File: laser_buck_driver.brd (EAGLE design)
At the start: 160 x 100 mm, 23 parts, among them IC1 LM358D, IC2 LM2576, SW1 TACT

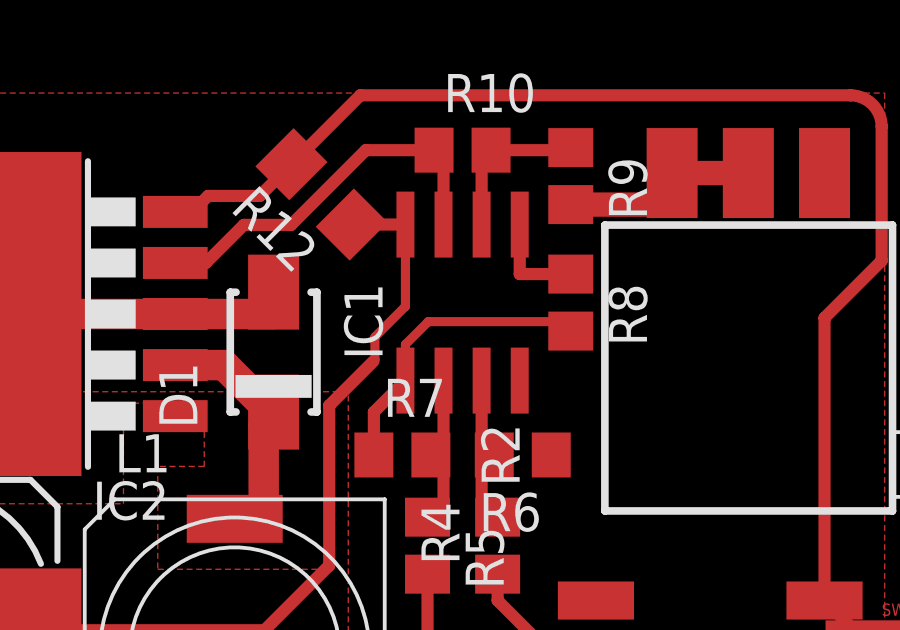
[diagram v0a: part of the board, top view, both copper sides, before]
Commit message: comments
screenshot and minor updates
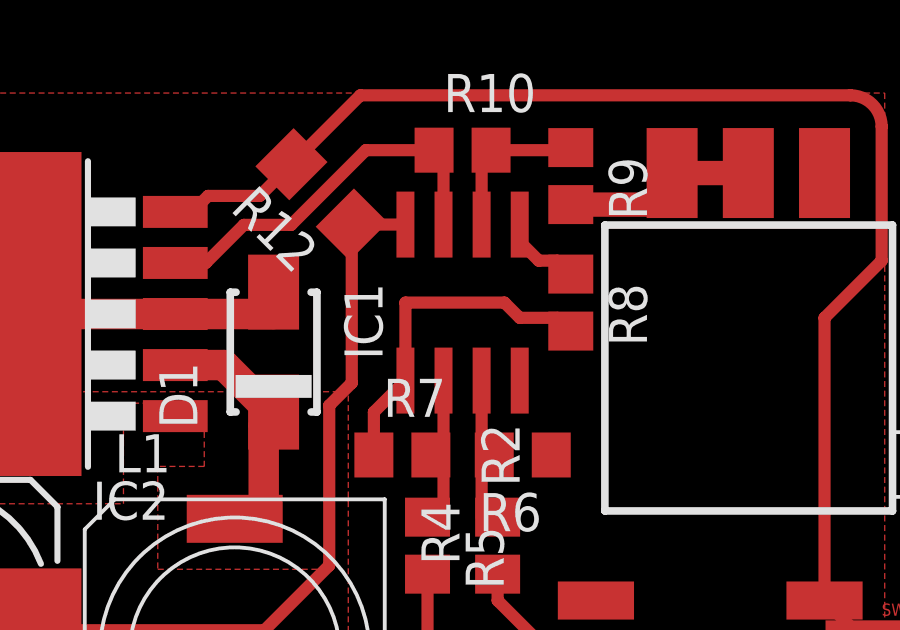
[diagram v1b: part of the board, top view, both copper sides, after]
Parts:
- R10: value 100k -> 470k
- R4, R5: value 22k -> 100k
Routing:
- net N$3: track 10.3 -> 11.7 mm
- net +18V: track 34.5 -> 33.7 mm
- net 22K: track 3.35 -> 2.72 mm
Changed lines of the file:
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@@
 <layer number="23" name="tOrigins" color="15" fill="1" visible="yes" active="yes"/>
 <layer number="24" name="bOrigins" color="15" fill="1" visible="yes" active="yes"/>
-<layer number="25" name="tNames" color="7" fill="1" visible="yes" active="yes"/>
-<layer number="26" name="bNames" color="7" fill="1" visible="yes" active="yes"/>
-<layer number="27" name="tValues" color="7" fill="1" visible="yes" active="yes"/>
-<layer number="28" name="bValues" color="7" fill="1" visible="yes" active="yes"/>
+<layer number="25" name="tNames" color="7" fill="1" visible="no" active="yes"/>
+<layer number="26" name="bNames" color="7" fill="1" visible="no" active="yes"/>
+<layer number="27" name="tValues" color="7" fill="1" visible="no" active="yes"/>
+<layer number="28" name="bValues" color="7" fill="1" visible="no" active="yes"/>
 <layer number="29" name="tStop" color="7" fill="3" visible="no" active="yes"/>
 <layer number="30" name="bStop" color="7" fill="6" visible="no" active="yes"/>
@@
 <rectangle x1="40.259" y1="41.1734" x2="43.6118" y2="44.0436" layer="41"/>
 <rectangle x1="35.179" y1="41.1734" x2="38.5318" y2="44.0436" layer="41"/>
-<dimension x1="71.5264" y1="66.675" x2="71.5264" y2="40.005" x3="78.105" y3="53.34" textsize="1.778" layer="51" dtype="vertical"/>
-<dimension x1="71.5264" y1="40.005" x2="31.6992" y2="40.005" x3="51.6128" y3="33.02" textsize="1.778" layer="51" dtype="vertical"/>
+<dimension x1="71.5264" y1="66.675" x2="71.5264" y2="40.005" x3="74.93" y3="53.34" textsize="1.778" layer="51" dtype="vertical"/>
+<dimension x1="71.5264" y1="40.005" x2="31.6992" y2="40.005" x3="51.6128" y3="36.83" textsize="1.778" layer="51" dtype="vertical"/>
 <wire x1="36.1188" y1="48.7934" x2="38.3286" y2="48.7934" width="0.3048" layer="41"/>
 </plain>
@@
 <element name="C2" library="rcl" package="153CLV-0810" value="100u/25V" x="38.1762" y="49.4538"/>
 <element name="R3" library="rcl" package="R1206" value="0.1R" x="56.8706" y="44.958" rot="R90"/>
-<element name="R4" library="rcl" package="R0805" value="22k" x="57.0484" y="51.4604" rot="R90"/>
-<element name="R5" library="rcl" package="R0805" value="22k" x="54.7116" y="51.4604" rot="R270"/>
+<element name="R4" library="rcl" package="R0805" value="100k" x="57.0484" y="51.4604" rot="R90"/>
+<element name="R5" library="rcl" package="R0805" value="100k" x="54.7116" y="51.4604" rot="R270"/>
 <element name="R6" library="rcl" package="R0805" value="100k" x="57.8866" y="54.483" rot="R180"/>
 <element name="R7" library="rcl" package="R0805" value="100k" x="53.8734" y="54.483"/>
 <element name="R8" library="rcl" package="R0805" value="20k/do_pominiecia" x="59.4868" y="59.563" rot="R270"/>
 <element name="R9" library="rcl" package="R0805" value="1k" x="59.4868" y="63.7794" rot="R270"/>
-<element name="R10" library="rcl" package="R0805" value="100k" x="55.88" y="64.643"/>
+<element name="R10" library="rcl" package="R0805" value="470k" x="55.88" y="64.643"/>
 <element name="SW1" library="miscrel" package="TACT" value="TACT" x="64.135" y="47.0916" rot="R90"/>
 <element name="R12" library="resistor" package="R1206" value="100k" x="51.181" y="63.1698" rot="R135"/>
@@
 <wire x1="52.9234" y1="55.9114" x2="52.9234" y2="54.483" width="0.4064" layer="1"/>
 <wire x1="59.4868" y1="58.928" x2="59.4868" y2="58.613" width="0.3048" layer="1"/>
-<wire x1="54.737" y1="58.928" x2="53.975" y2="58.166" width="0.3048" layer="1"/>
-<wire x1="53.975" y1="58.166" x2="53.975" y2="56.963" width="0.3048" layer="1"/>
-<wire x1="59.4868" y1="58.928" x2="54.737" y2="58.928" width="0.3048" layer="1"/>
+<wire x1="53.975" y1="56.963" x2="53.975" y2="59.563" width="0.4064" layer="1"/>
+<wire x1="53.975" y1="59.563" x2="57.277" y2="59.563" width="0.4064" layer="1"/>
+<wire x1="57.277" y1="59.563" x2="57.785" y2="59.055" width="0.4064" layer="1"/>
+<wire x1="57.785" y1="59.055" x2="59.0448" y2="59.055" width="0.4064" layer="1"/>
+<wire x1="59.0448" y1="59.055" x2="59.4868" y2="58.613" width="0.4064" layer="1"/>
 </signal>
 <signal name="N$12">
@@
 <contactref element="R8" pad="1"/>
 <contactref element="IC1" pad="5"/>
-<wire x1="57.785" y1="62.163" x2="57.785" y2="60.513" width="0.4064" layer="1"/>
-<wire x1="57.785" y1="60.513" x2="59.4868" y2="60.513" width="0.4064" layer="1"/>
+<wire x1="57.785" y1="62.163" x2="57.785" y2="61.595" width="0.4064" layer="1"/>
+<wire x1="57.785" y1="61.595" x2="58.42" y2="60.96" width="0.4064" layer="1"/>
+<wire x1="58.42" y1="60.96" x2="59.0398" y2="60.96" width="0.4064" layer="1"/>
+<wire x1="59.0398" y1="60.96" x2="59.4868" y2="60.513" width="0.4064" layer="1"/>
 </signal>
 <signal name="N$15">
@@
 <wire x1="46.3042" y1="59.182" x2="49.5808" y2="59.182" width="1.016" layer="1"/>
 <wire x1="49.5808" y1="59.182" x2="49.5808" y2="59.912" width="1.016" layer="1"/>
-<wire x1="49.5808" y1="59.182" x2="57.785" y2="56.963" width="0" layer="19" extent="1-1"/>
+<wire x1="57.785" y1="56.963" x2="49.5808" y2="59.182" width="0" layer="19" extent="1-1"/>
 </signal>
 <signal name="+18V">
@@
 <contactref element="IC2" pad="1"/>
 <contactref element="PAD1" pad="1"/>
-<wire x1="53.975" y1="62.163" x2="53.975" y2="59.436" width="0.3048" layer="1"/>
-<wire x1="53.975" y1="59.436" x2="52.959" y2="58.42" width="0.3048" layer="1"/>
-<wire x1="52.959" y1="58.42" x2="52.959" y2="57.658" width="0.3048" layer="1"/>
-<wire x1="52.959" y1="57.658" x2="52.9082" y2="57.6072" width="0.3048" layer="1"/>
-<wire x1="52.9082" y1="57.6072" x2="51.435" y2="56.134" width="0.4064" layer="1"/>
 <wire x1="51.435" y1="56.134" x2="51.435" y2="50.8" width="0.4064" layer="1"/>
 <wire x1="51.435" y1="50.8" x2="49.276" y2="48.641" width="0.4064" layer="1"/>
@@
 </polygon>
 <wire x1="36.8554" y1="43.307" x2="36.8554" y2="45.7454" width="1.27" layer="1"/>
+<wire x1="51.435" y1="56.134" x2="52.186503125" y2="56.885503125" width="0.4064" layer="1"/>
+<wire x1="52.186503125" y1="56.885503125" x2="52.186503125" y2="62.16429375" width="0.4064" layer="1"/>
 </signal>
 <signal name="N$2">
